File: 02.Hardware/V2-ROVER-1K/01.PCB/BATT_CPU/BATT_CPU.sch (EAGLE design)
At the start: 70 parts, among them K2 FLEX12, Q1 BSS84W-7-F, Q2 BSS84W-7-F, Q3 2N7002PW, Q4 2N7002PW, Q5 BSS84W-7-F, U1 ATSAMD21G18_QFN, U3 TPS78230DDCR, U6 MAX9062EUK+T, U8 SN74LVC1G19DBVR, X2 32.768

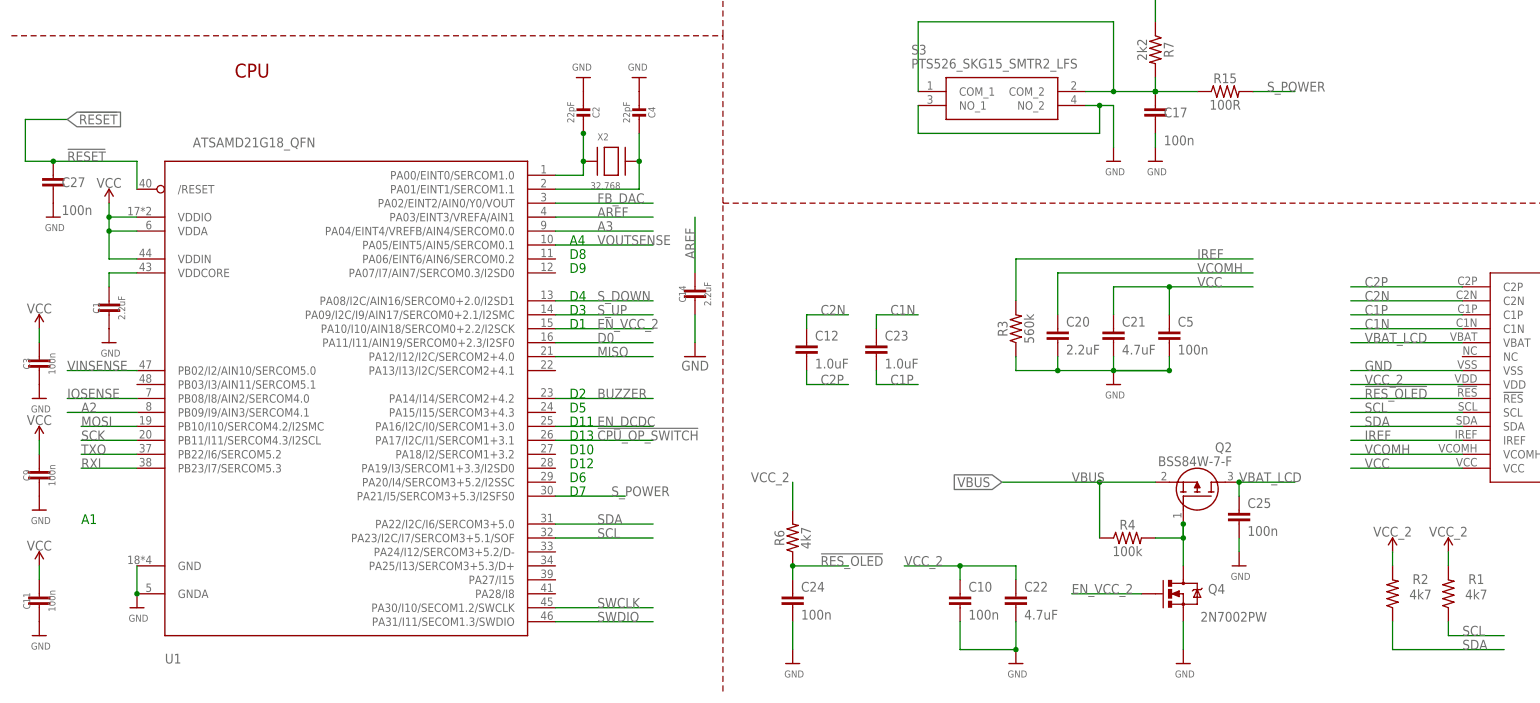
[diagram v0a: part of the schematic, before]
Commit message: Revision antes de enviar a SETI
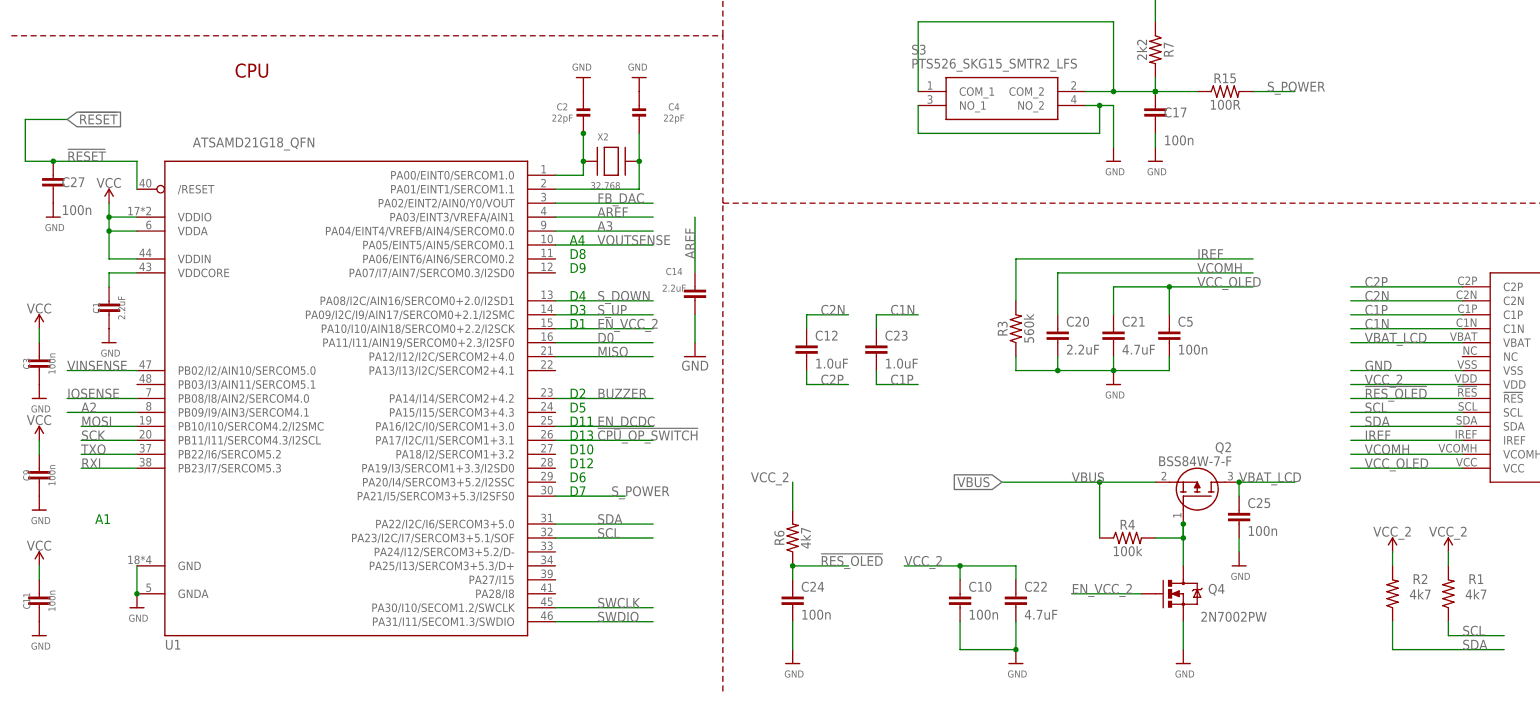
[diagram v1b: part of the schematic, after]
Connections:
- new net VCC_OLED: C21.1, C5.1, U$30.VCC
- net VCC: no longer C21.1, C5.1, U$30.VCC
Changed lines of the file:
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@@
 <text x="106.68" y="45.72" size="1.778" layer="91">D10</text>
 <text x="106.68" y="55.88" size="1.778" layer="91">D2</text>
-<text x="17.78" y="33.02" size="1.778" layer="91">A1</text>
+<text x="20.32" y="33.02" size="1.778" layer="91">A1</text>
 <wire x1="134.62" y1="167.64" x2="261.62" y2="167.64" width="0.1524" layer="94" style="shortdash"/>
 <text x="276.86" y="246.38" size="2.54" layer="94">CHARGING DETECTOR
@@
 </instance>
 <instance part="C14" gate="G$1" x="129.54" y="73.66" smashed="yes">
-<attribute name="NAME" x="127.25" y="74.91" size="1.27" layer="95" font="vector" rot="R90" align="center"/>
-<attribute name="VALUE" x="131.84" y="74.91" size="1.27" layer="96" font="vector" rot="R90" align="center"/>
+<attribute name="NAME" x="125.75" y="78.99" size="1.27" layer="95" font="vector" rot="R180" align="center"/>
+<attribute name="VALUE" x="125.75" y="75.96" size="1.27" layer="96" font="vector" rot="R180" align="center"/>
 </instance>
 <instance part="U$34" gate="G$1" x="297.18" y="17.78" smashed="yes"/>
 <instance part="U$35" gate="G$1" x="292.1" y="17.78" smashed="yes"/>
 <instance part="U1" gate="G$1" x="53.34" y="60.96" smashed="yes">
-<attribute name="NAME" x="33.02" y="7.62" size="1.778" layer="95"/>
+<attribute name="NAME" x="33.02" y="10.16" size="1.778" layer="95"/>
 <attribute name="VALUE" x="38.1" y="101.6" size="1.778" layer="96"/>
 </instance>
@@
 </instance>
 <instance part="C2" gate="G$1" x="109.22" y="109.22" smashed="yes" rot="R180">
-<attribute name="NAME" x="111.51" y="107.97" size="1.27" layer="95" font="vector" rot="R270" align="center"/>
-<attribute name="VALUE" x="106.92" y="107.97" size="1.27" layer="96" font="vector" rot="R270" align="center"/>
+<attribute name="NAME" x="105.39" y="108.97" size="1.27" layer="95" font="vector" align="center"/>
+<attribute name="VALUE" x="105.39" y="106.92" size="1.27" layer="96" font="vector" align="center"/>
 </instance>
 <instance part="C4" gate="G$1" x="119.38" y="109.22" smashed="yes" rot="R180">
-<attribute name="NAME" x="121.67" y="107.97" size="1.27" layer="95" font="vector" rot="R270" align="center"/>
-<attribute name="VALUE" x="117.08" y="107.97" size="1.27" layer="96" font="vector" rot="R270" align="center"/>
+<attribute name="NAME" x="125.71" y="108.97" size="1.27" layer="95" font="vector" align="center"/>
+<attribute name="VALUE" x="125.71" y="106.92" size="1.27" layer="96" font="vector" align="center"/>
 </instance>
 <instance part="U$8" gate="G$1" x="109.22" y="114.3" smashed="yes" rot="R180">
@@
 <wire x1="187.96" y1="60.96" x2="195.58" y2="60.96" width="0.1524" layer="91"/>
 <pinref part="C21" gate="G$1" pin="2"/>
-<wire x1="195.58" y1="60.96" x2="215.9" y2="60.96" width="0.1524" layer="91"/>
+<wire x1="195.58" y1="60.96" x2="205.74" y2="60.96" width="0.1524" layer="91"/>
 <wire x1="215.9" y1="60.96" x2="205.74" y2="60.96" width="0.1524" layer="91"/>
 <wire x1="205.74" y1="60.96" x2="205.74" y2="63.5" width="0.1524" layer="91"/>
@@
 <pinref part="C5" gate="G$1" pin="2"/>
 <wire x1="215.9" y1="63.5" x2="215.9" y2="60.96" width="0.1524" layer="91"/>
-<junction x="215.9" y="60.96"/>
 <pinref part="U$9" gate="G$1" pin="GND"/>
 <pinref part="C20" gate="G$1" pin="2"/>
@@
 </segment>
 <segment>
-<pinref part="U$30" gate="G$1" pin="VCC"/>
-<wire x1="269.24" y1="43.18" x2="248.92" y2="43.18" width="0.1524" layer="91"/>
-<label x="251.46" y="43.18" size="1.778" layer="95"/>
-</segment>
-<segment>
-<wire x1="205.74" y1="76.2" x2="215.9" y2="76.2" width="0.1524" layer="91"/>
-<label x="220.98" y="76.2" size="1.778" layer="95"/>
-<pinref part="C21" gate="G$1" pin="1"/>
-<wire x1="205.74" y1="76.2" x2="205.74" y2="71.12" width="0.1524" layer="91"/>
-<pinref part="C5" gate="G$1" pin="1"/>
-<wire x1="215.9" y1="71.12" x2="215.9" y2="76.2" width="0.1524" layer="91"/>
-<wire x1="215.9" y1="76.2" x2="231.14" y2="76.2" width="0.1524" layer="91"/>
-<junction x="215.9" y="76.2"/>
-</segment>
-<segment>
 <pinref part="R48" gate="G$1" pin="2"/>
 <pinref part="SUPPLY11" gate="G$1" pin="VCC"/>
@@
 </segment>
 </net>
+<net name="VCC_OLED" class="0">
+<segment>
+<wire x1="205.74" y1="76.2" x2="215.9" y2="76.2" width="0.1524" layer="91"/>
+<label x="220.98" y="76.2" size="1.778" layer="95"/>
+<pinref part="C21" gate="G$1" pin="1"/>
+<wire x1="205.74" y1="76.2" x2="205.74" y2="71.12" width="0.1524" layer="91"/>
+<pinref part="C5" gate="G$1" pin="1"/>
+<wire x1="215.9" y1="71.12" x2="215.9" y2="76.2" width="0.1524" layer="91"/>
+<wire x1="215.9" y1="76.2" x2="231.14" y2="76.2" width="0.1524" layer="91"/>
+<junction x="215.9" y="76.2"/>
+</segment>
+<segment>
+<pinref part="U$30" gate="G$1" pin="VCC"/>
+<wire x1="269.24" y1="43.18" x2="248.92" y2="43.18" width="0.1524" layer="91"/>
+<label x="251.46" y="43.18" size="1.778" layer="95"/>
+</segment>
+</net>
